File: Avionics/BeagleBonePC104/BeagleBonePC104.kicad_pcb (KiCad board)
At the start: 2 copper layers, 4 parts

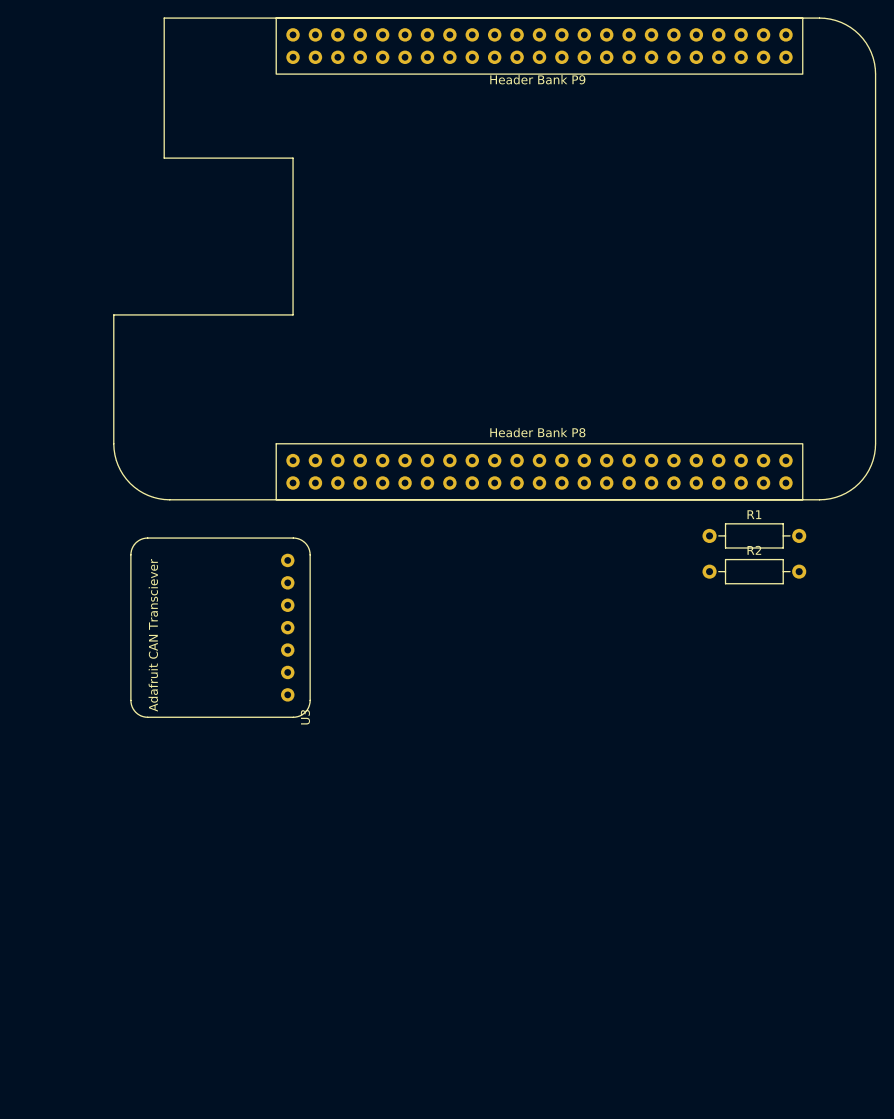
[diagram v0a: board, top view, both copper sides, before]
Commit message: Ian Goldberg - Finished the footprint for the BeagleBonePCI104 Motherboard
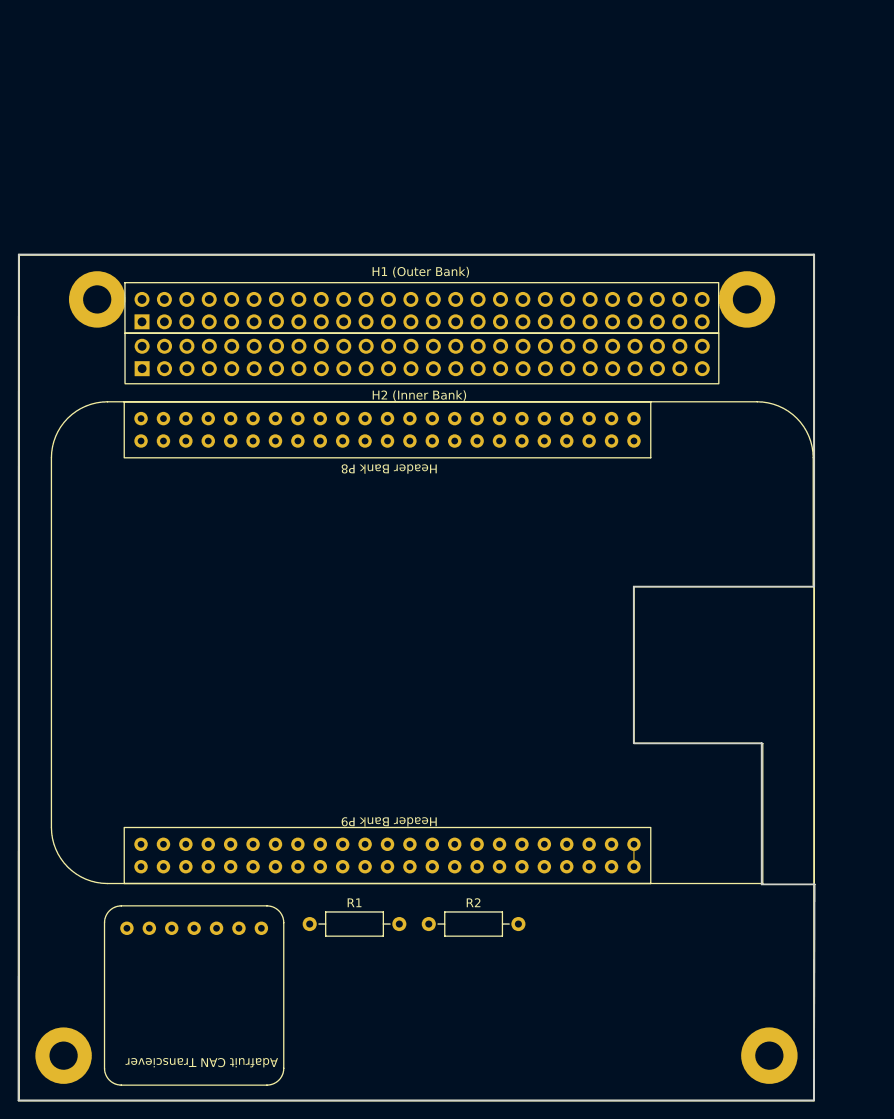
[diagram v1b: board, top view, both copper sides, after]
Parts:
- added U2: ~, PCI104Connector:PCI104ConnectorAttempt#2H1, F.Cu at (80.0, 170.0)
- added U4: ~, PCI104Connector:PCI104ConnectorAttempt#2H2, F.Cu at (80.0, 170.0)
- moved U1 80.1 mm to (170.1, 90.8), turned to 180 degrees
- moved R1 63.2 mm to (113.0, 150.0)
- moved R2 51.1 mm to (126.5, 150.0)
- moved U3 21.6 mm to (110.1, 147.9), turned to 180 degrees
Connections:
- U1 pad 25: /GPIO3_21 -> /CAN_SLNT
- U3 pad 1: (no net) -> /3V3
- U3 pad 2: (no net) -> GND
- U3 pad 3: (no net) -> /CAN1_TX
- U3 pad 4: (no net) -> /CAN1_RX
- U3 pad 5: (no net) -> /CAN_SLNT
- U3 pad 6: (no net) -> /CAN_H
- U3 pad 7: (no net) -> /CAN_L
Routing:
- net GND: track 0.00 -> 2.54 mm
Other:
- board outline added: 90.2 x 95.9 mm
